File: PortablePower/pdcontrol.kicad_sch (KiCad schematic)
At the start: 32 parts, among them IC1 SW6208, J1 USB1130-15-A, J2 2137160001, Q1 CSD17313Q2, Q2 CSD17313Q2, U1 USBLC6-2SC6, U2 USBLC6-2SC6

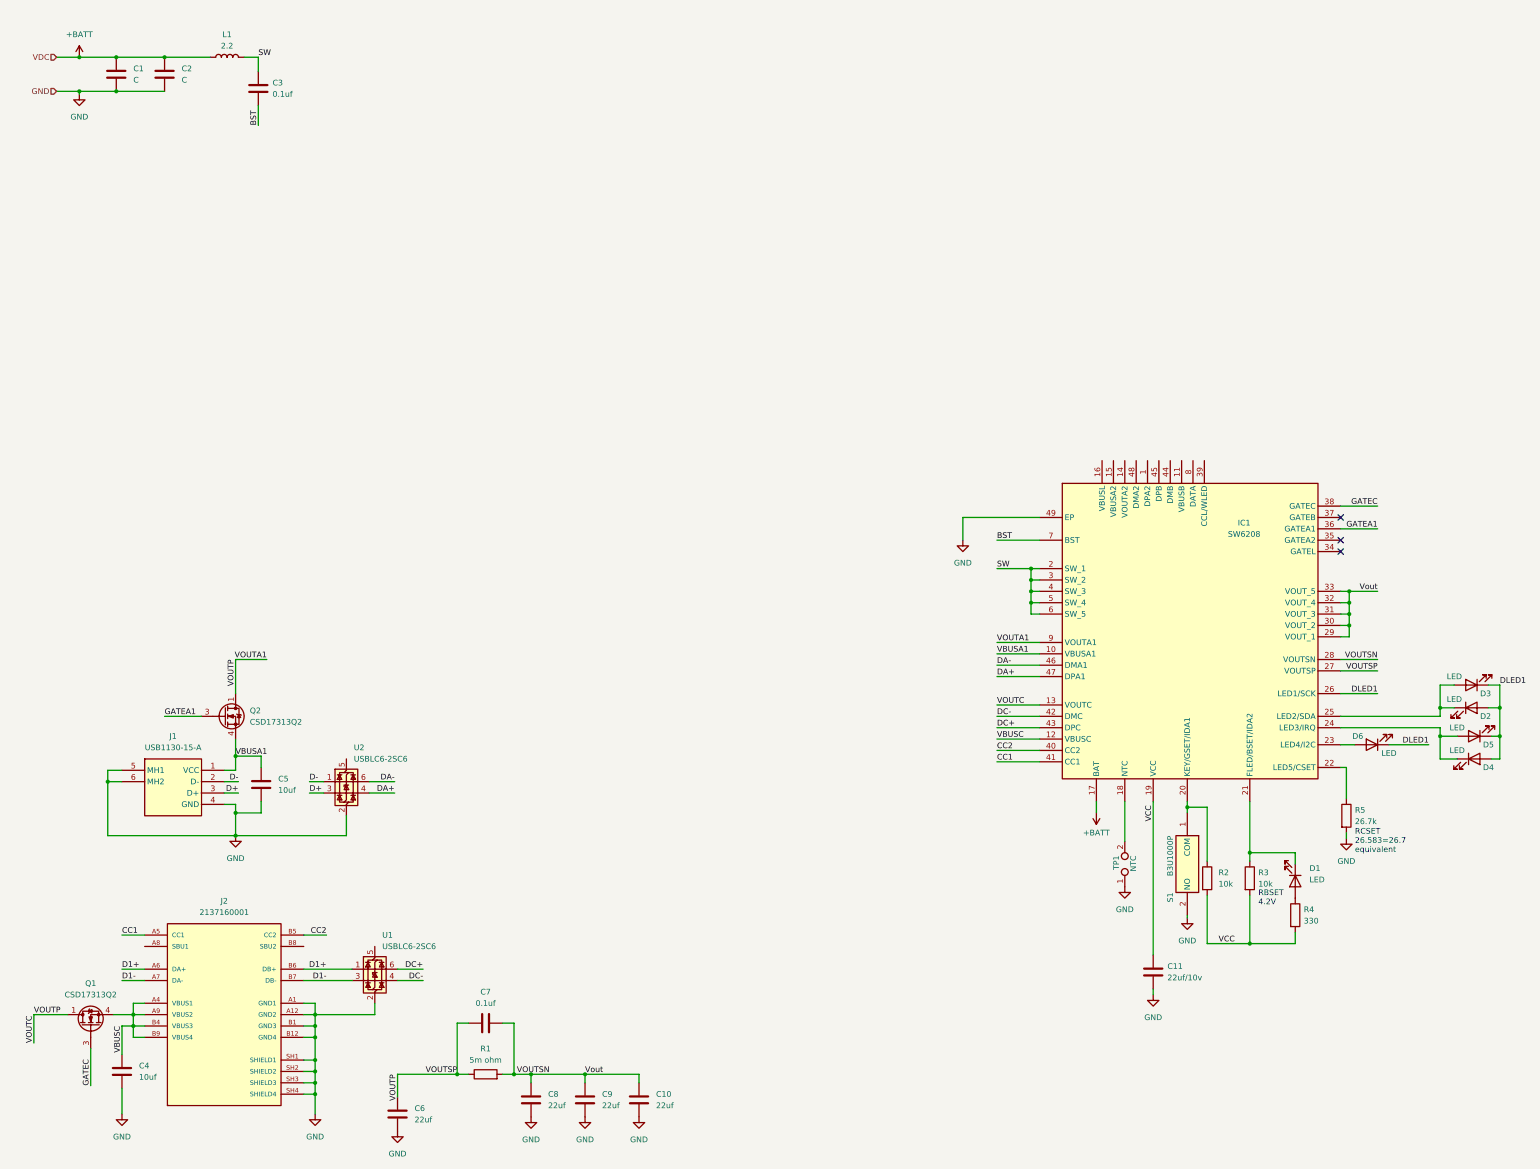
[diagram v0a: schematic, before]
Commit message: schematic complete
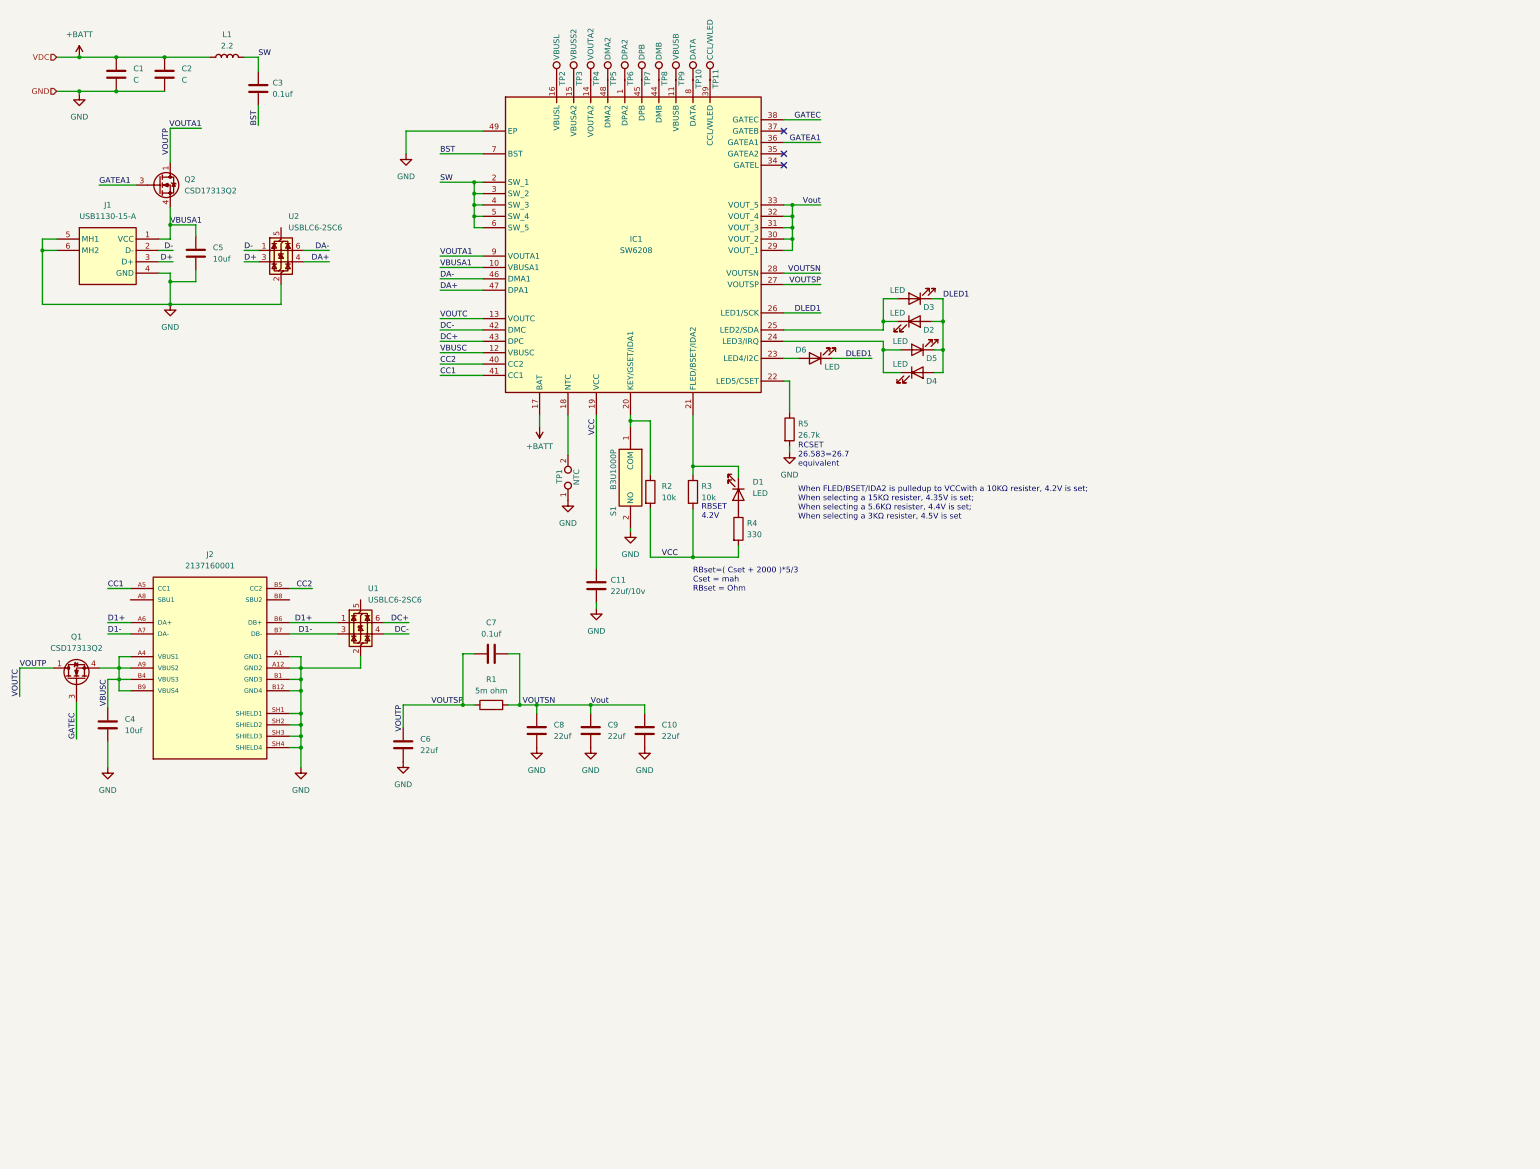
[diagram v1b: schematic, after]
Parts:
- added TP10: DATA, TestPoint:TestPoint_Pad_D1.0mm, symbol Connector:TestPoint
- added TP11: CCL/WLED, TestPoint:TestPoint_Pad_D1.0mm, symbol Connector:TestPoint
- added TP2: VBUSL, TestPoint:TestPoint_Pad_D1.0mm, symbol Connector:TestPoint
- added TP3: VBUSS2, TestPoint:TestPoint_Pad_D1.0mm, symbol Connector:TestPoint
- added TP4: VOUTA2, TestPoint:TestPoint_Pad_D1.0mm, symbol Connector:TestPoint
- added TP5: DMA2, TestPoint:TestPoint_Pad_D1.0mm, symbol Connector:TestPoint
- added TP6: DPA2, TestPoint:TestPoint_Pad_D1.0mm, symbol Connector:TestPoint
- added TP7: DPB, TestPoint:TestPoint_Pad_D1.0mm, symbol Connector:TestPoint
- added TP8: DMB, TestPoint:TestPoint_Pad_D1.0mm, symbol Connector:TestPoint
- added TP9: VBUSB, TestPoint:TestPoint_Pad_D1.0mm, symbol Connector:TestPoint
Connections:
- net at IC1.1 (DPA2): now also TP6.1
- net at IC1.11 (VBUSB): now also TP9.1
- net at IC1.14 (VOUTA2): now also TP4.1
- net at IC1.15 (VBUSA2): now also TP3.1
- net at IC1.16 (VBUSL): now also TP2.1
- net at IC1.39 (CCL/WLED): now also TP11.1
- net at IC1.44 (DMB): now also TP8.1
- net at IC1.45 (DPB): now also TP7.1
- net at IC1.48 (DMA2): now also TP5.1
- net at IC1.8 (DATA): now also TP10.1
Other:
- note added: "RBset=( Cset + 2000 )*5/3 Cset = mah RBset = Ohm"
- note added: "When FLED/BSET/IDA2 is pulledup to VCCwith a 10KΩ resister, 4.2V is set; When selecting a 15KΩ resister, 4.35V is set; When selecting a 5.6KΩ resister, 4.4V is set; When selecting a 3KΩ resister, 4.5V is set"
- moved on the sheet: C10, C11, C4, C5, C6, C7, C8, C9, D1, D2, D3, D4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
